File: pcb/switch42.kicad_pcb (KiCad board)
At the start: 2 copper layers, 128.6 x 66.7 mm, 43 parts, among them J1 MJ-4PP-9, SW1 SW_PUSH, SW10 SW_PUSH, SW11 SW_PUSH, SW12 SW_PUSH, SW13 SW_PUSH, SW14 SW_PUSH, SW15 SW_PUSH, SW16 SW_PUSH, SW17 SW_PUSH, SW18 SW_PUSH, SW19 SW_PUSH, SW2 SW_PUSH, SW3 SW_PUSH, SW4 SW_PUSH, SW5 SW_PUSH, SW6 SW_PUSH, SW7 SW_PUSH, SW8 SW_PUSH, SW9 SW_PUSH, U1 ProMicro

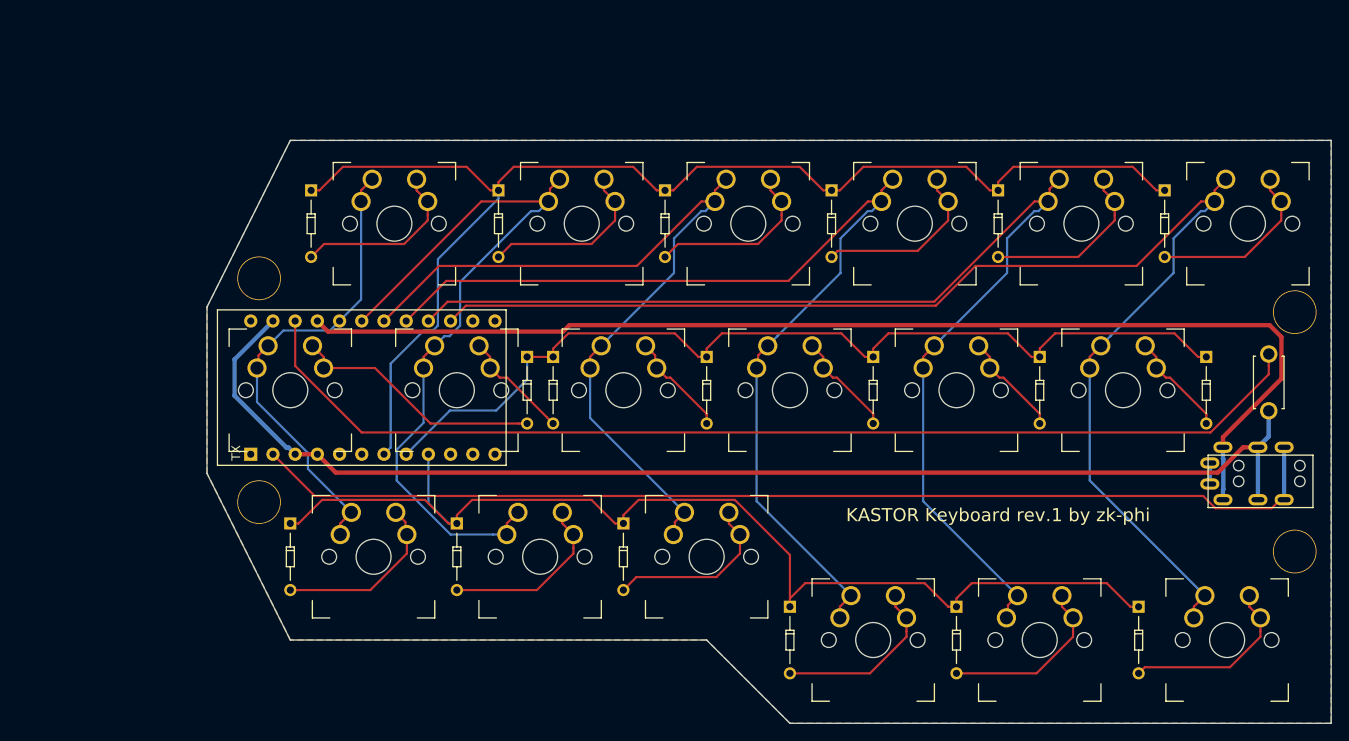
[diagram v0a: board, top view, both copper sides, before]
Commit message: Redraw schema and update pcb layout
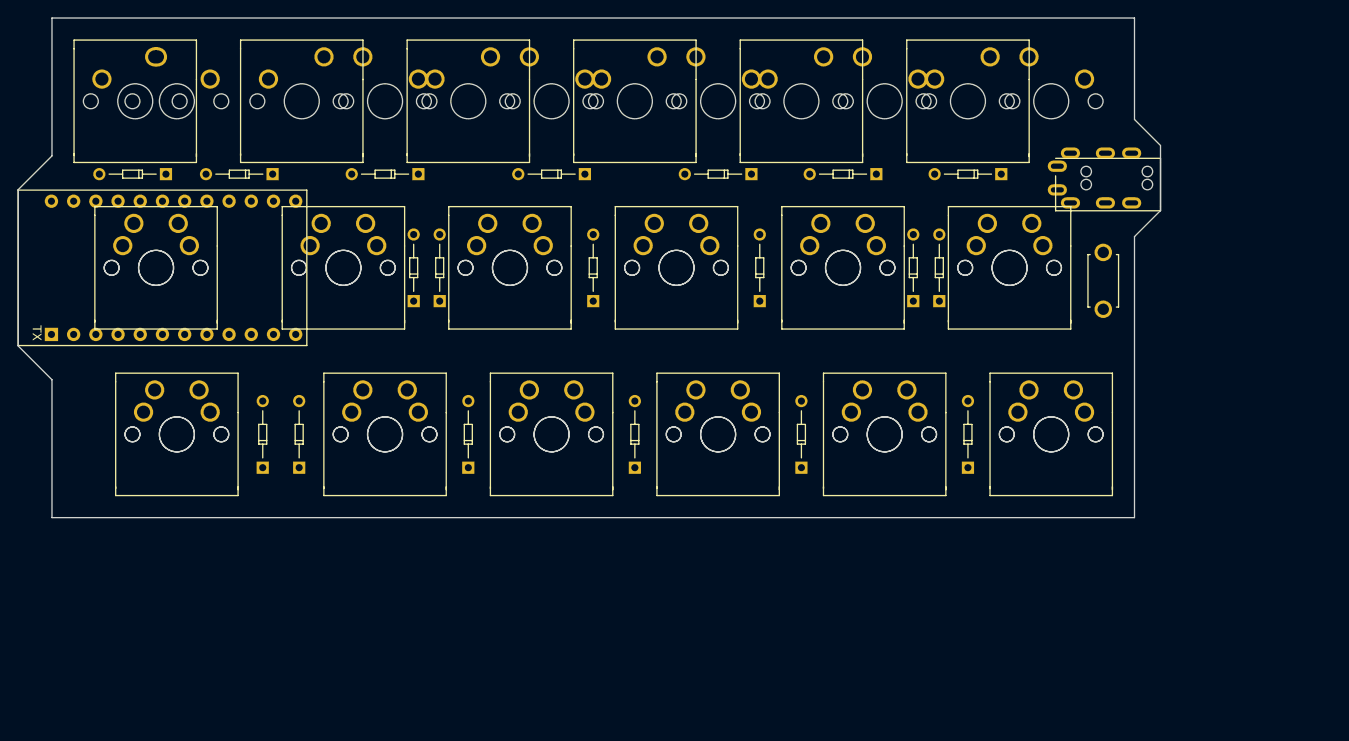
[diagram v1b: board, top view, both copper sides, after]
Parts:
- removed Ref** (x4): Val**, phi-kbd-library:M2_SPACER_HOLE
- added D19: D, phi-kbd-library:D_TH-reversible, F.Cu at (156.0, 52.9)
- added J2: MJ-4PP-9, phi-kbd-library:MJ-4PP-9-irreversible, B.Cu at (178.0, 52.6)
- added SW20: SW_PUSH, phi-kbd-library:MX_1.00u-irreversible, B.Cu at (165.5, 44.6)
- added SW21: SW_PUSH, phi-kbd-library:MX_1.25u-irreversible, B.Cu at (63.1, 63.6)
- added SW22: SW_PUSH, phi-kbd-library:MX_1.50u-irreversible, B.Cu at (65.5, 82.7)
- added SW23: SW_PUSH, phi-kbd-library:MX_1.50u-irreversible, B.Cu at (65.5, 44.6)
- added SW24: SW_PUSH, phi-kbd-library:MX_1.00u-irreversible, B.Cu at (84.6, 63.6)
- added SW25: SW_PUSH, phi-kbd-library:MX_1.00u-irreversible, B.Cu at (89.3, 82.7)
- added SW26: SW_PUSH, phi-kbd-library:MX_1.00u-irreversible, B.Cu at (89.3, 44.6)
- added SW27: SW_PUSH, phi-kbd-library:MX_1.00u-irreversible, B.Cu at (103.6, 63.6)
- added SW28: SW_PUSH, phi-kbd-library:MX_1.00u-irreversible, B.Cu at (108.4, 82.7)
- added SW29: SW_PUSH, phi-kbd-library:MX_1.00u-irreversible, B.Cu at (108.4, 44.6)
- added SW30: SW_PUSH, phi-kbd-library:MX_1.00u-irreversible, B.Cu at (122.7, 63.6)
- added SW31: SW_PUSH, phi-kbd-library:MX_1.00u-irreversible, B.Cu at (127.4, 82.7)
- added SW32: SW_PUSH, phi-kbd-library:MX_1.00u-irreversible, B.Cu at (127.4, 44.6)
- added SW33: SW_PUSH, phi-kbd-library:MX_1.00u-irreversible, B.Cu at (141.7, 63.6)
- added SW34: SW_PUSH, phi-kbd-library:MX_1.00u-irreversible, B.Cu at (146.5, 82.7)
- added SW35: SW_PUSH, phi-kbd-library:MX_1.00u-irreversible, B.Cu at (146.5, 44.6)
- added SW36: SW_PUSH, phi-kbd-library:MX_1.00u-irreversible, B.Cu at (160.8, 63.6)
- added SW37: SW_PUSH, phi-kbd-library:MX_1.00u-irreversible, B.Cu at (165.5, 82.7)
- J1: footprint phi-kbd-library:MJ-4PP-9-reversible -> phi-kbd-library:MJ-4PP-9-irreversible; moved to F.Cu
- SW10, SW11, SW12, SW13, SW14, SW15, SW16, SW17, SW18, SW5, SW6, SW7, SW8, SW9: footprint phi-kbd-library:MX_1.00u-reversible -> phi-kbd-library:MX_1.00u-irreversible
- SW19, SW2: footprint phi-kbd-library:MX_1.25u-reversible -> phi-kbd-library:MX_1.00u-irreversible
- SW3: footprint phi-kbd-library:MX_1.00u-reversible -> phi-kbd-library:MX_1.25u-irreversible
- SW4: footprint phi-kbd-library:MX_1.00u-reversible -> phi-kbd-library:MX_1.50u-irreversible
- moved J1 37.4 mm to (178.0, 54.1)
- moved D16 37.2 mm to (141.7, 52.9), turned to 180 degrees
- moved SW14 35.0 mm to (137.0, 44.6)
- moved SW17 35.0 mm to (156.0, 44.6)
- moved SW5 35.0 mm to (79.8, 44.6)
- moved SW8 35.0 mm to (98.9, 44.6)
- moved SW11 35.0 mm to (117.9, 44.6)
- moved D17 33.6 mm to (152.7, 63.6), turned to 90 degrees
- moved SW2 32.8 mm to (60.8, 44.6)
- moved D10 32.5 mm to (108.4, 52.9), turned to 180 degrees
- moved D13 32.5 mm to (127.4, 52.9), turned to 180 degrees
- moved D7 32.5 mm to (89.3, 52.9), turned to 180 degrees
- moved SW19 31.0 mm to (165.5, 82.7)
- moved D18 30.6 mm to (156.0, 82.7), turned to 90 degrees
- moved D4 30.2 mm to (72.7, 52.9), turned to 180 degrees
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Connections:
- net row3 renamed Net-(U1-Pad10)
- U1 pad 14: Net-(U1-Pad14) -> col6
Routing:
- net col5: track 155.9 -> 0.00 mm
- net row0: track 146.1 -> 0.00 mm
- net GND: track 143.0 -> 0.00 mm
- net col4: track 138.4 -> 0.00 mm
- net VCC: track 133.1 -> 0.00 mm
- net row2: track 126.7 -> 0.00 mm
- net reset: track 124.7 -> 0.00 mm
- net data: track 124.6 -> 0.00 mm
- net col3: track 121.9 -> 0.00 mm
- net row1: track 108.8 -> 0.00 mm
- net col2: track 95.9 -> 0.00 mm
- net col1: track 88.3 -> 0.00 mm
- net col0: track 54.2 -> 0.00 mm
- net Net-(D2-Pad2): track 29.0 -> 0.00 mm
- net Net-(D18-Pad2): track 20.9 -> 0.00 mm
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- removed copper zone on B.Cu, net GND
- removed copper zone on F.Cu, net GND
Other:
- board size 128.6 x 66.7 mm -> 130.7 x 57.2 mm
- board text removed: "KASTOR Keyboard rev.1 by zk-phi"
